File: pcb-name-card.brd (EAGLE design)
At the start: 87.5 x 54 mm, 7 parts

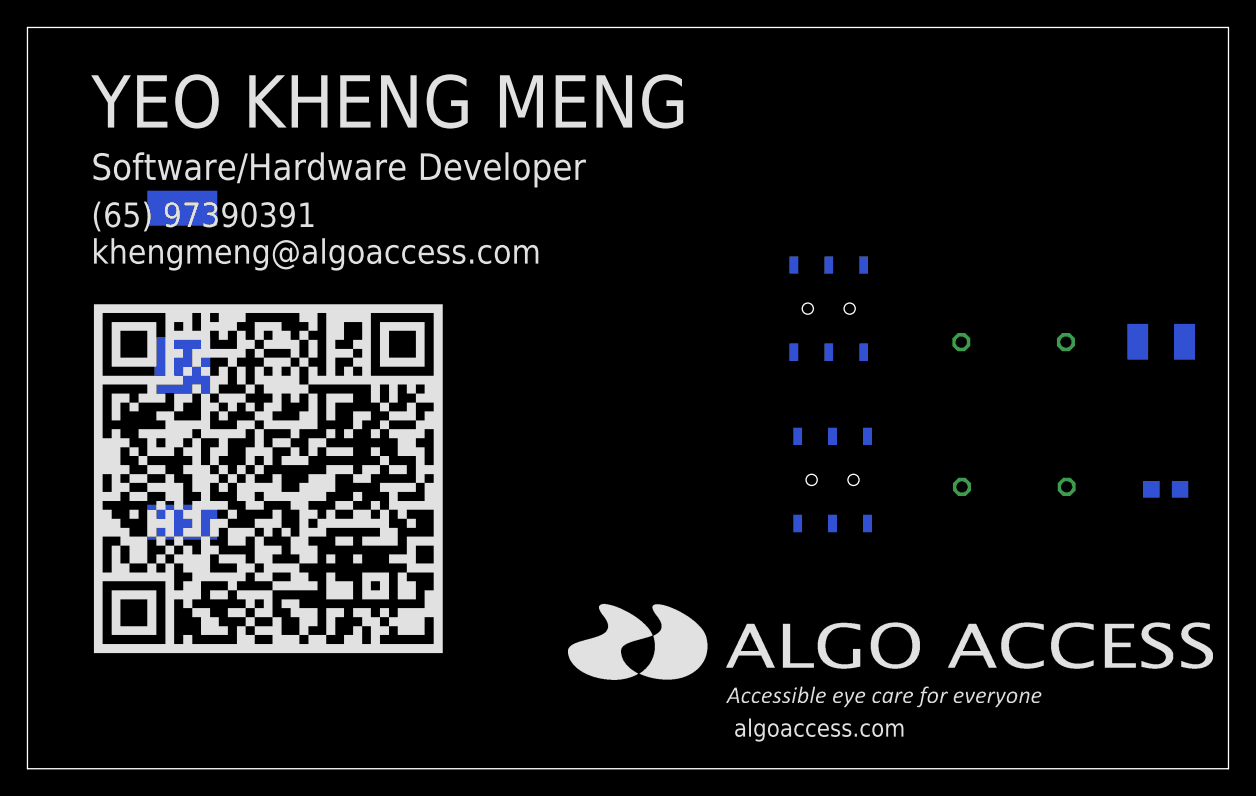
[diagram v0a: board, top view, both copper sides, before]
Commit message: aa banner
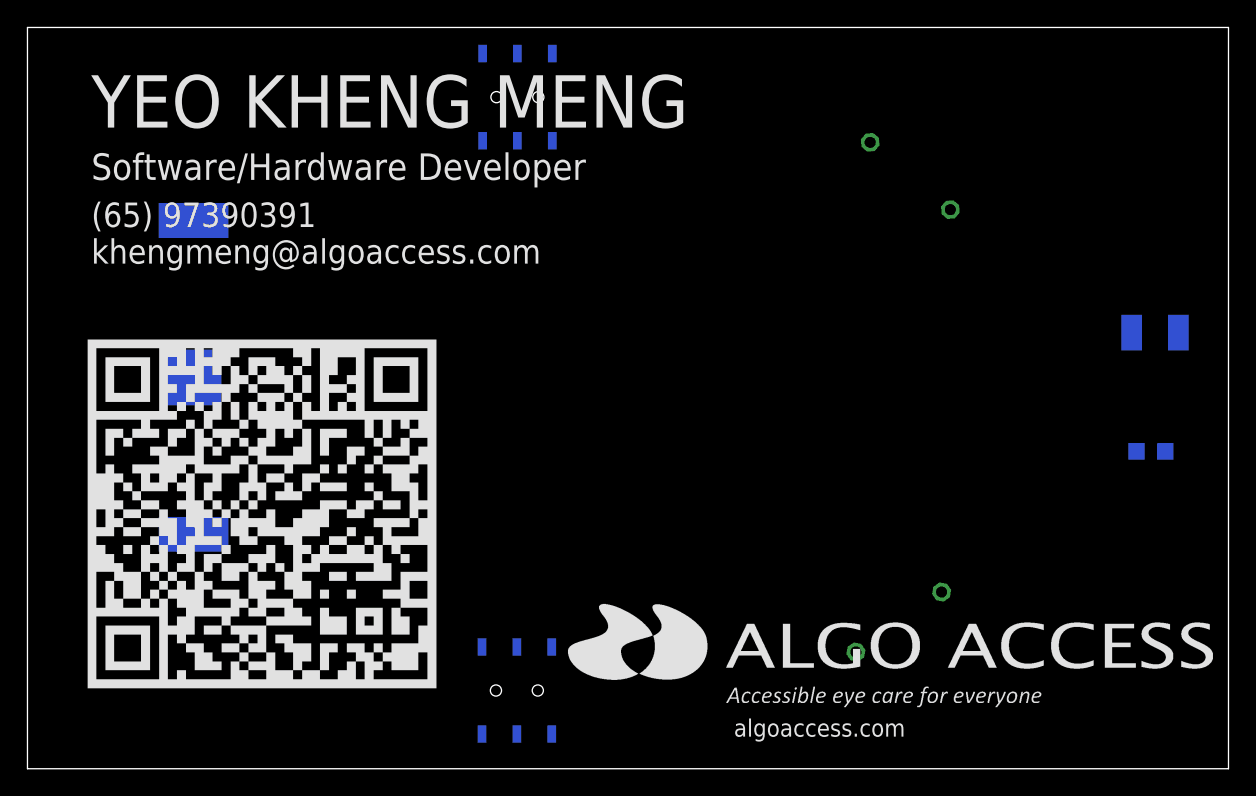
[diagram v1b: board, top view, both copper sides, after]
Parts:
- moved SW2 27.6 mm to (35.6, 5.70)
- moved SW1 27.4 mm to (35.7, 48.9)
- moved R1 14.2 mm to (64.3, 43.2), turned to 220 degrees
- moved R2 12.9 mm to (63.4, 10.7), turned to 145 degrees
- moved LED2 2.97 mm to (81.8, 23.1)
- moved U$1 1.21 mm to (12.1, 28.5)
- moved LED1 0.80 mm to (82.1, 31.8)
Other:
- board text added: "E:/Dropbox/git-projects/pcb-name-card/algoaccess banner.bmp"

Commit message: more changes
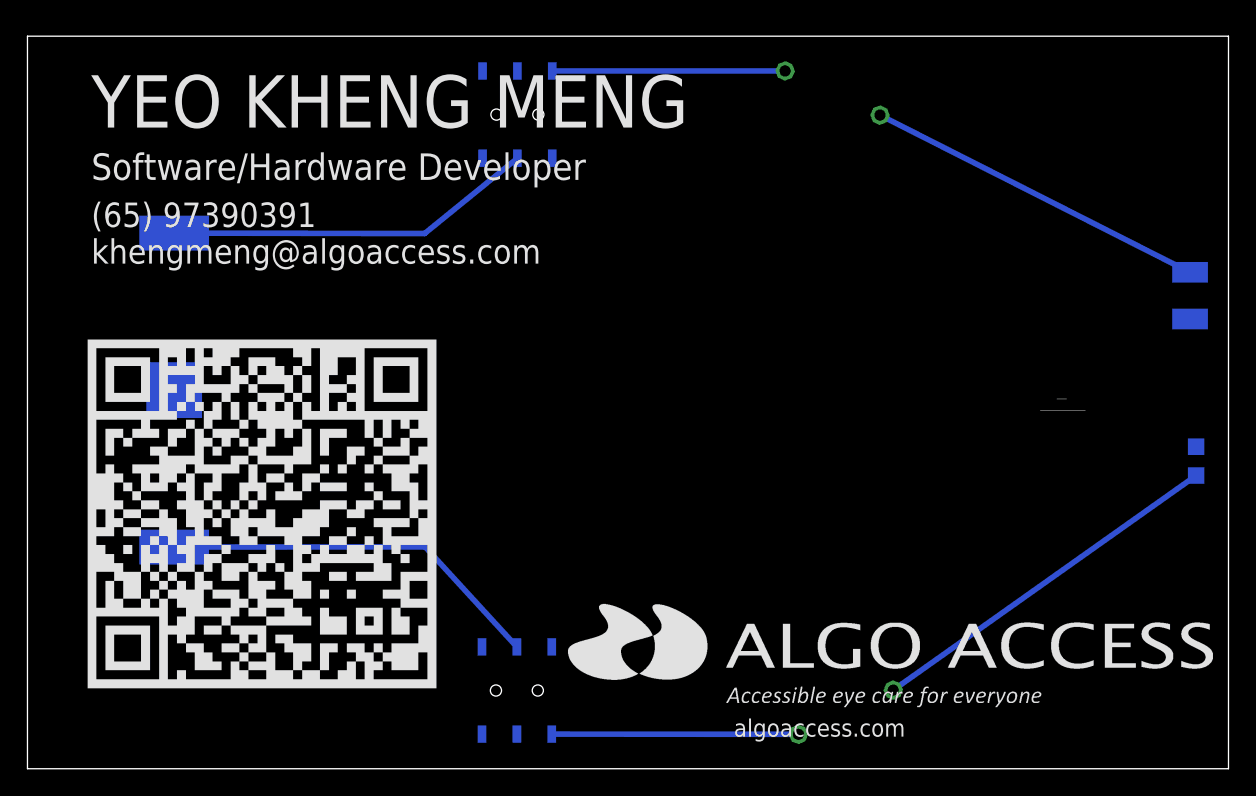
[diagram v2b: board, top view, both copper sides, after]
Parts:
- moved R1 8.28 mm to (58.6, 49.2), turned to 25 degrees
- moved R2 7.61 mm to (59.6, 4.11), turned to 335 degrees
- moved LED1 3.71 mm to (84.7, 34.4), turned to 0 degrees
- moved LED2 3.37 mm to (85.1, 22.4), turned to 0 degrees
- moved U$1 1.69 mm to (10.7, 27.6)
- moved SW1 1.27 mm to (35.7, 47.6)
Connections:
- net N$3: now also SW1.COM1; no longer SW1.COM2, U$1.+$2
- net N$4: now also SW1.CH2A; no longer SW1.CH1A
- net N$7: now also U$1.+$2; no longer SW1.COM1
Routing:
- net N$7: track 0.00 -> 28.2 mm
- net N$2: track 0.00 -> 27.0 mm
- net N$3: track 0.00 -> 26.9 mm
- net N$1: track 0.00 -> 25.3 mm
- net N$5: track 0.00 -> 18.0 mm
- net N$4: track 0.00 -> 17.0 mm
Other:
- board size 87.5 x 54 mm -> 87.5 x 53.3 mm
- board text added: "E:/Dropbox/git-projects/pcb-name-card/algoaccess banner mirror.bmp"

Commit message: some changes
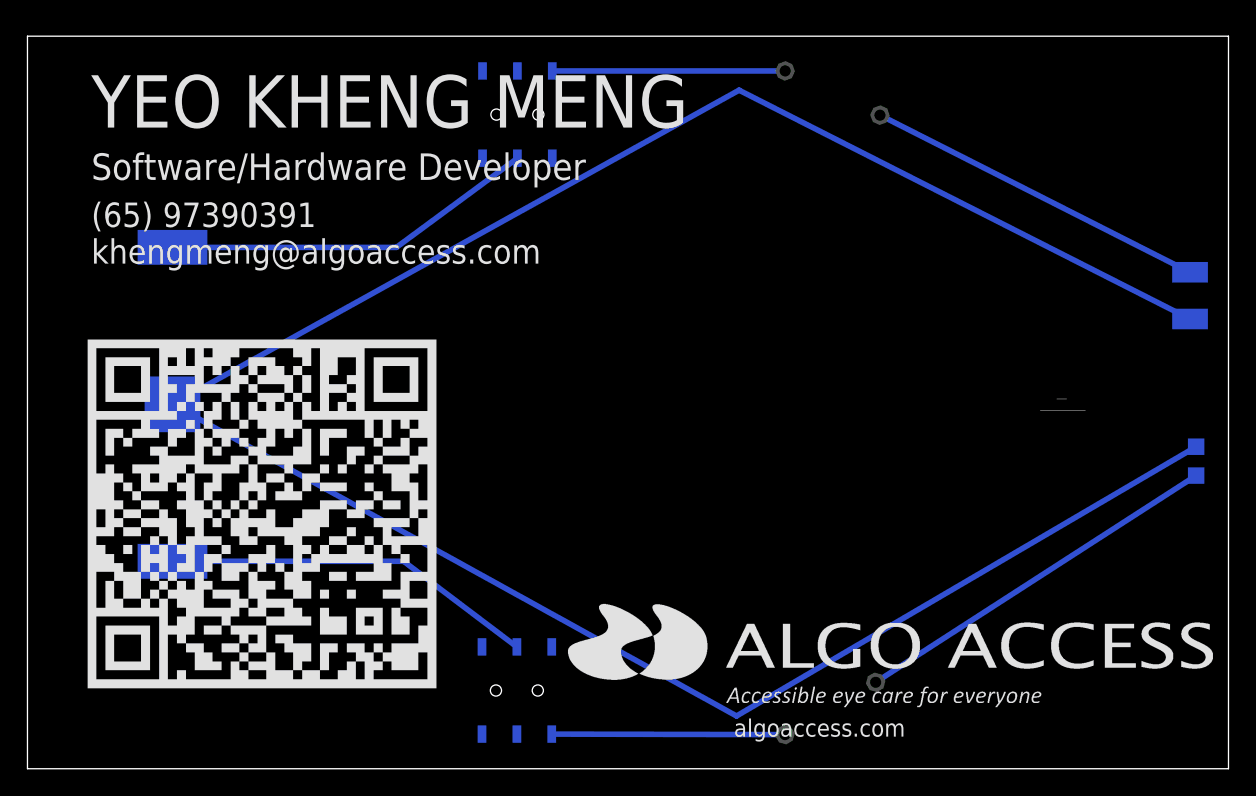
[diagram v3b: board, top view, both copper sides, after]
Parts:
- moved R2 1.16 mm to (58.5, 4.39), turned to 330 degrees
- moved U$1 1.04 mm to (10.6, 26.5)
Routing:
- net N$6: track 0.00 -> 169.7 mm
- net N$7: track 28.2 -> 27.2 mm
- net N$5: track 18.0 -> 17.0 mm
- net N$2: track 27.0 -> 27.8 mm
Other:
- board text added: "Caution: Look away from LEDs before toggling the switches"
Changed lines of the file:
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@@
 <layer number="26" name="bNames" color="7" fill="1" visible="yes" active="yes"/>
 <layer number="27" name="tValues" color="7" fill="1" visible="no" active="yes"/>
-<layer number="28" name="bValues" color="7" fill="1" visible="no" active="yes"/>
+<layer number="28" name="bValues" color="7" fill="1" visible="yes" active="yes"/>
 <layer number="29" name="tStop" color="7" fill="3" visible="no" active="yes"/>
 <layer number="30" name="bStop" color="7" fill="6" visible="no" active="yes"/>
@@
 <layer number="43" name="vRestrict" color="2" fill="10" visible="no" active="yes"/>
 <layer number="44" name="Drills" color="7" fill="1" visible="no" active="yes"/>
-<layer number="45" name="Holes" color="7" fill="1" visible="yes" active="yes"/>
-<layer number="46" name="Milling" color="3" fill="1" visible="yes" active="yes"/>
+<layer number="45" name="Holes" color="7" fill="1" visible="no" active="yes"/>
+<layer number="46" name="Milling" color="3" fill="1" visible="no" active="yes"/>
 <layer number="47" name="Measures" color="7" fill="1" visible="no" active="yes"/>
 <layer number="48" name="Document" color="7" fill="1" visible="no" active="yes"/>
@@
 <layer number="120" name="KAP_MAAT1" color="7" fill="1" visible="no" active="no"/>
 <layer number="121" name="_tsilk" color="7" fill="1" visible="no" active="yes"/>
-<layer number="122" name="_bsilk" color="7" fill="1" visible="no" active="yes"/>
+<layer number="122" name="_bsilk" color="7" fill="1" visible="yes" active="yes"/>
 <layer number="123" name="tTestmark" color="7" fill="1" visible="no" active="yes"/>
 <layer number="124" name="bTestmark" color="7" fill="1" visible="no" active="yes"/>
@@
 <rectangle x1="53.29428125" y1="46.0400375" x2="53.721" y2="46.0705125" layer="22"/>
 <text x="0" y="-0.1524" size="0.060959375" layer="22" font="vector" rot="MR0">E:/Dropbox/git-projects/pcb-name-card/algoaccess banner mirror.bmp</text>
+<text x="30.9372" y="4.693921875" size="1.27" layer="22" font="vector" rot="MR0">Caution: Look away from LEDs
+before toggling the switches</text>
 </plain>
 <attributes>
@@
 <element name="LED1" library="led" package="PLCC2" value="UV" x="84.65185" y="34.44875" smashed="yes" rot="MR0">
 <attribute name="COLOR" value="yellow" x="84.65185" y="34.44875" size="1.778" layer="28" rot="MR0" display="off"/>
-<attribute name="VALUE" x="80.84185" y="32.54375" size="1.27" layer="28" rot="MR90"/>
+<attribute name="VALUE" x="80.84185" y="33.214309375" size="1.27" layer="28" rot="MR90"/>
 </element>
 <element name="LED2" library="led" package="CHIP-LED0805" value="Light" x="85.09635" y="22.39645" smashed="yes" rot="MR0">
-<attribute name="VALUE" x="81.9531" y="19.8247" size="1.27" layer="28" rot="MR90"/>
+<attribute name="VALUE" x="82.0140625" y="19.5808625" size="1.27" layer="28" rot="MR90"/>
 </element>
-<element name="U$1" library="cr2032" package="CR2032-SMD" value="" x="10.6807" y="27.570428125" smashed="yes" rot="MR270">
-<attribute name="VALUE" x="23.0307" y="31.888428125" size="1.6764" layer="28" font="vector" rot="MR270"/>
+<element name="U$1" library="cr2032" package="CR2032-SMD" value="" x="10.558778125" y="26.534109375" smashed="yes" rot="MR270">
+<attribute name="VALUE" x="22.908778125" y="30.852109375" size="1.6764" layer="28" font="vector" rot="MR270"/>
 </element>
 <element name="SW1" library="Seeed-OPL-Switch" package="SW6-2.54-SMD-7.0X3.5X1.5MM" value="" x="35.6743" y="47.63135" smashed="yes" rot="MR90">
@@
 </element>
 <element name="R1" library="resistor" package="0207/7" value="" x="58.6232" y="49.1998" smashed="yes" rot="MR25">
-<attribute name="NAME" x="59.17851875" y="48.488415625" size="1.27" layer="26" ratio="10" rot="MR25"/>
+<attribute name="NAME" x="59.239478125" y="48.244575" size="1.27" layer="26" ratio="10" rot="MR25"/>
 <attribute name="VALUE" x="60.458859375" y="47.72725" size="1.27" layer="28" ratio="10" rot="MR25"/>
 </element>
-<element name="R2" library="resistor" package="0207/7" value="" x="59.5884" y="4.1148" smashed="yes" rot="MR335">
-<attribute name="NAME" x="60.47875625" y="3.87030625" size="1.27" layer="26" ratio="10" rot="MR335"/>
-<attribute name="VALUE" x="61.89638125" y="4.5744625" size="1.27" layer="28" ratio="10" rot="MR335"/>
+<element name="R2" library="resistor" package="0207/7" value="" x="58.460640625" y="4.38911875" smashed="yes" rot="MR330">
+<attribute name="NAME" x="59.368915625" y="4.223153125" size="1.27" layer="26" ratio="10" rot="MR330"/>
+<attribute name="VALUE" x="60.719775" y="5.048184375" size="1.27" layer="28" ratio="10" rot="MR330"/>
 </element>
 </elements>
@@
 <contactref element="R2" pad="1"/>
 <contactref element="LED2" pad="A"/>
-<wire x1="63.041434375" y1="5.724975" x2="85.09635" y2="21.34645" width="0.4064" layer="16"/>
+<wire x1="61.7602" y1="6.29411875" x2="85.09635" y2="21.34645" width="0.4064" layer="16"/>
 </signal>
 <signal name="N$6">
@@
 <contactref element="LED1" pad="C"/>
 <contactref element="LED2" pad="C"/>
-<wire x1="85.09635" y1="23.44645" x2="84.65185" y2="32.74875" width="0" layer="19" extent="16-16"/>
-<wire x1="10.6807" y1="27.570428125" x2="84.65185" y2="32.74875" width="0" layer="19" extent="16-16"/>
+<wire x1="84.65185" y1="32.74875" x2="51.816" y2="49.408078125" width="0.4064" layer="16"/>
+<wire x1="51.816" y1="49.408078125" x2="10.558778125" y2="26.534109375" width="0.4064" layer="16"/>
+<wire x1="85.09635" y1="23.44645" x2="51.63311875" y2="3.84048125" width="0.4064" layer="16"/>
+<wire x1="51.63311875" y1="3.84048125" x2="10.558778125" y2="26.534109375" width="0.4064" layer="16"/>
 </signal>
 <signal name="N$3">
 <contactref element="U$1" pad="+$1"/>
 <contactref element="SW1" pad="COM1"/>
-<wire x1="10.6807" y1="39.000428125" x2="28.9179" y2="38.96995" width="0.4064" layer="16"/>
-<wire x1="28.9179" y1="38.96995" x2="35.6743" y2="44.45635" width="0.4064" layer="16"/>
+<wire x1="10.558778125" y1="37.964109375" x2="26.86558125" y2="37.964109375" width="0.4064" layer="16"/>
+<wire x1="26.86558125" y1="37.964109375" x2="35.6743" y2="44.45635" width="0.4064" layer="16"/>
 </signal>
 <signal name="N$7">
 <contactref element="U$1" pad="+$2"/>
 <contactref element="SW2" pad="COM2"/>
-<wire x1="10.6807" y1="16.140428125" x2="28.956" y2="16.1544" width="0.4064" layer="16"/>
-<wire x1="28.956" y1="16.1544" x2="35.6362" y2="8.87095" width="0.4064" layer="16"/>
+<wire x1="10.558778125" y1="15.104109375" x2="27.3913625" y2="15.104109375" width="0.4064" layer="16"/>
+<wire x1="27.3913625" y1="15.104109375" x2="35.6362" y2="8.87095" width="0.4064" layer="16"/>
 </signal>
 <signal name="N$5">
 <contactref element="R2" pad="2"/>
 <contactref element="SW2" pad="CH1A"/>
-<wire x1="56.13536875" y1="2.504621875" x2="38.1762" y2="2.52095" width="0.4064" layer="16"/>
+<wire x1="55.161084375" y1="2.484115625" x2="38.1762" y2="2.52095" width="0.4064" layer="16"/>
 </signal>
 <signal name="N$4">

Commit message: some updates
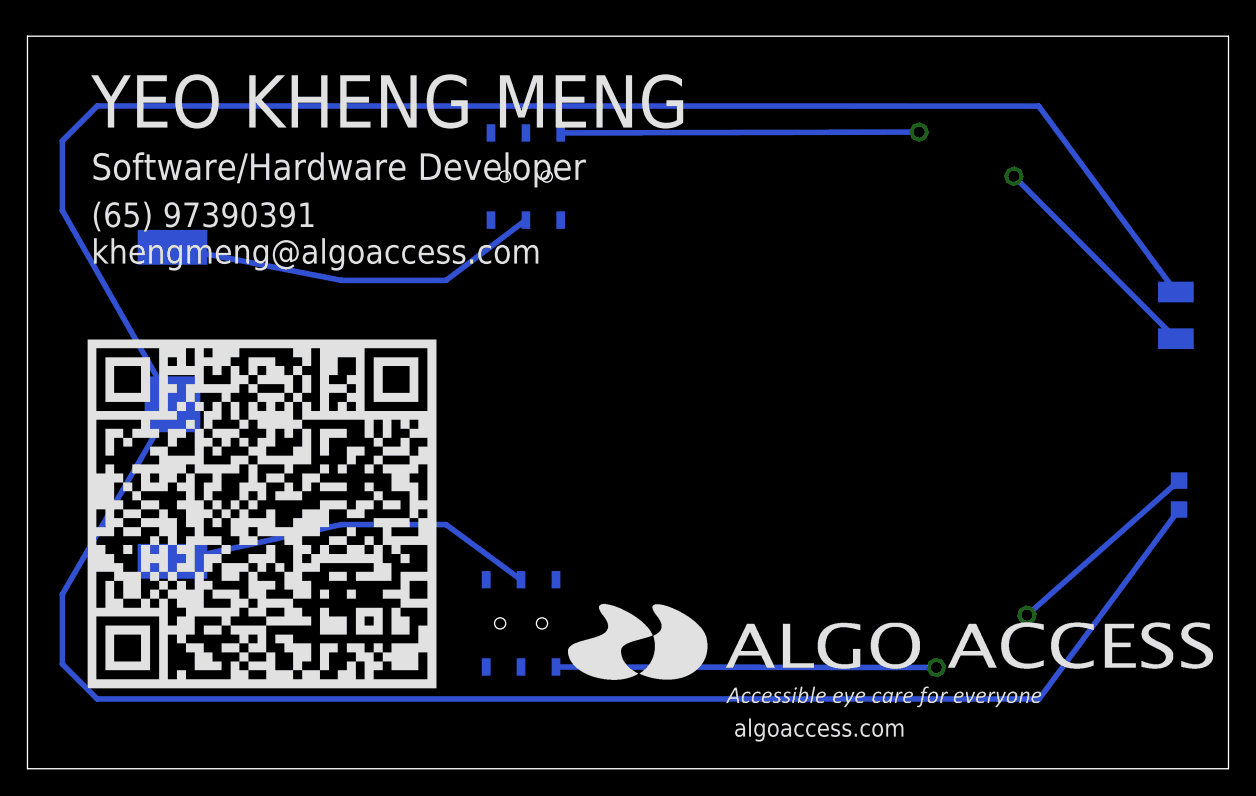
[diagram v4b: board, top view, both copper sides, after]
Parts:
- moved R2 12.1 mm to (69.5, 9.28)
- moved R1 10.7 mm to (68.4, 44.7)
- moved SW2 4.90 mm to (35.9, 10.6)
- moved SW1 4.55 mm to (36.3, 43.1)
- moved LED2 2.77 mm to (83.9, 19.9), turned to 180 degrees
- moved LED1 1.77 mm to (83.6, 33.0), turned to 180 degrees
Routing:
- net N$6: track 169.7 -> 220.7 mm
- net N$2: track 27.8 -> 14.8 mm
- net N$5: track 17.0 -> 27.7 mm
- net N$4: track 17.0 -> 26.1 mm
- net N$1: track 25.3 -> 16.7 mm
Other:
- board text added: "CR2025"
